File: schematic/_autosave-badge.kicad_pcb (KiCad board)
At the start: 2 copper layers, 90.2 x 45.7 mm, 50 parts, among them J1 Left2, J10 Left1, J11 Penny2, J12 Penny1, J13 Penny0, J14 Power, J15 Right5, J2 Left3, J4 Serial, J5 Penny3, J6 Right1, J7 Right2, J9 Right4, U1 ESP32-WROOM

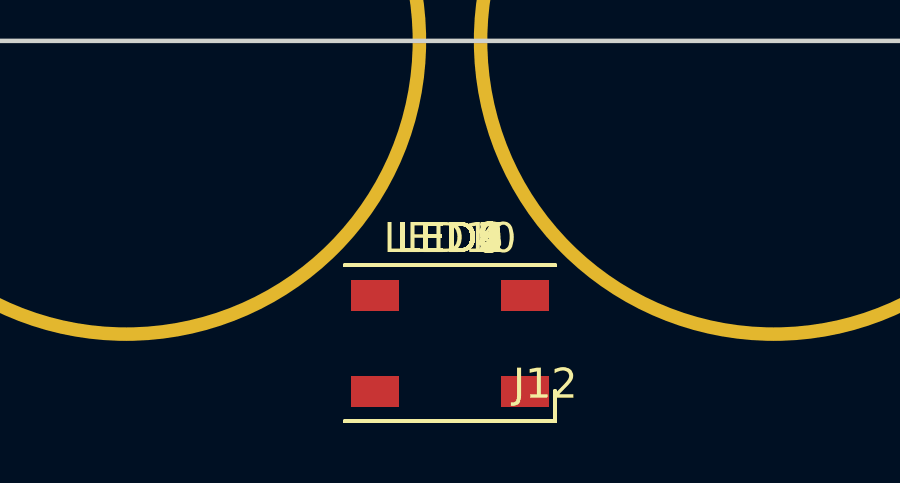
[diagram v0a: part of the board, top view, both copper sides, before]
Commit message: Checking for update
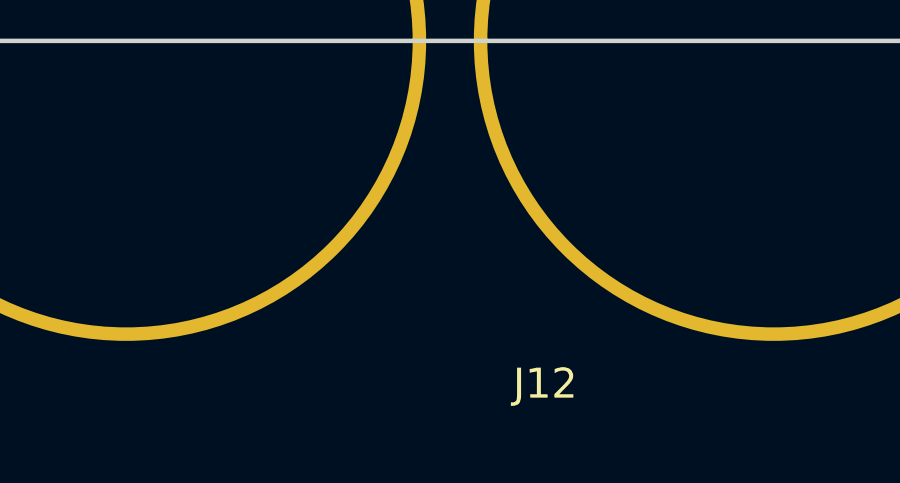
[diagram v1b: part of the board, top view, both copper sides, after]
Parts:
- removed LED1, LED10, LED2, LED3, LED4, LED5, LED6, LED7, LED8, LED9: WS2812B, LEDs:LED_WS2812B-PLCC4
